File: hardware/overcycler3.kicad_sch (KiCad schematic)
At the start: 97 parts, among them J10 Control_Down, J2 AudioJack3_Switch, J3 DIN-5_180degree, J4 AudioJack3_Switch, J5 AudioJack3_Switch, J6 Control_Up, J7 Keyboard, J8 Display, J9 FT232, Q1 2SC945, SW1 RESET, U1 XT26G02CWSIGA, U2 TL064, U3 LPC1778FBD144, U4 TLV2556, U5 74HC138, U6 TL064, Y1 12MHz

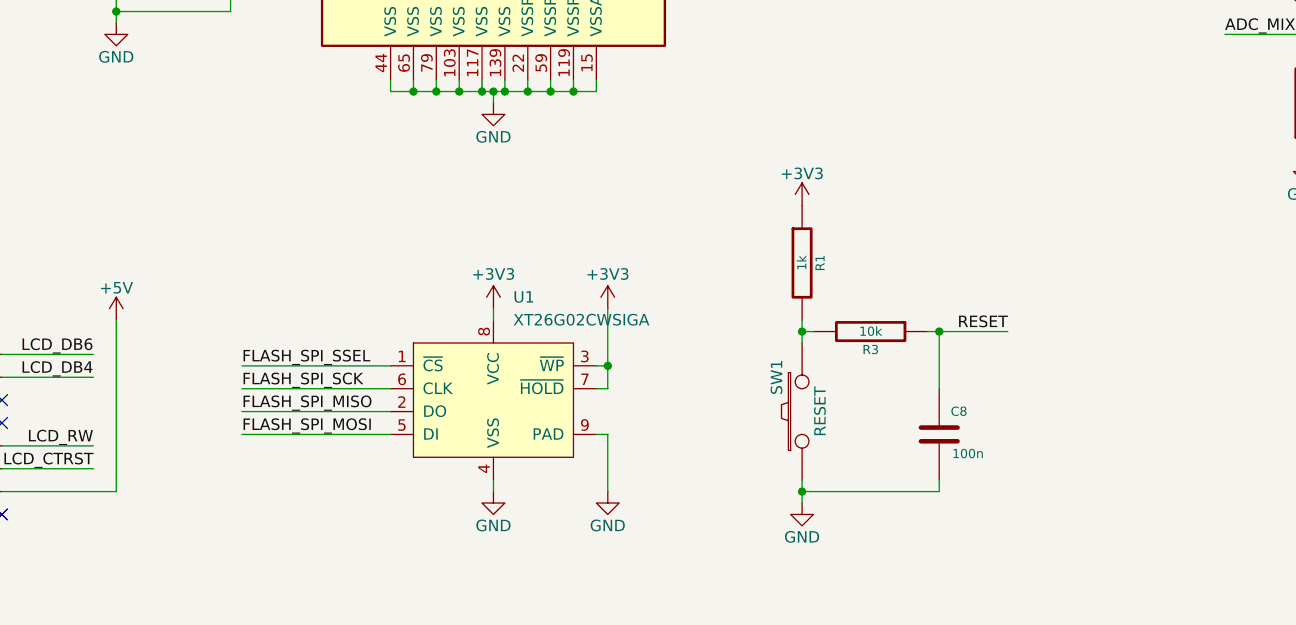
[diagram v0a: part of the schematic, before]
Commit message: sch: NAND -> 512Mb NOR FLASH
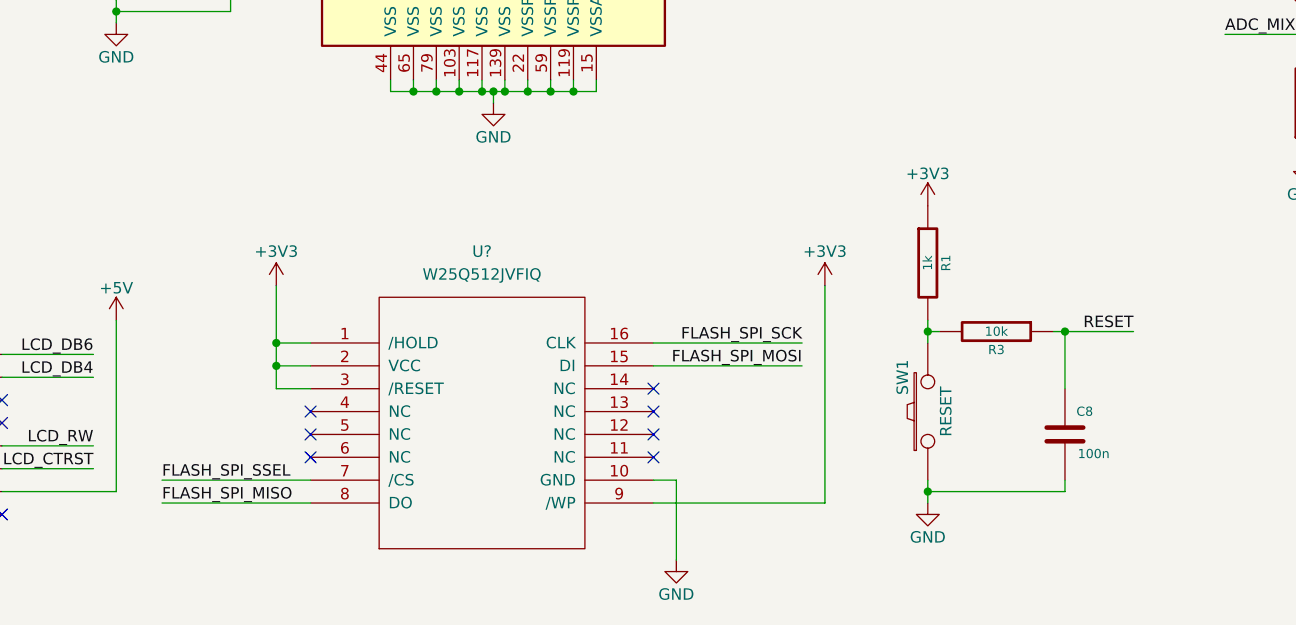
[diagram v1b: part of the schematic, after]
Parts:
- removed U1: XT26G02CWSIGA, Package_SON:WSON-8-1EP_8x6mm_P1.27mm_EP3.4x4.3mm, symbol Additional:XT26G02ELGIGA
- added U?: W25Q512JVFIQ, Package_SO:SOIC-16W_7.5x10.3mm_P1.27mm, symbol W25Q512JVFIQ:W25Q512JVFIQ
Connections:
- net +3V3: now also U?.1 (/HOLD), U?.2 (VCC), U?.3 (/RESET), U?.9 (/WP)
- net FLASH_SPI_MISO: now also U?.8 (DO)
- net FLASH_SPI_MOSI: now also U?.15 (DI)
- net FLASH_SPI_SCK: now also U?.16 (CLK)
- net FLASH_SPI_SSEL: now also U?.7 (/CS)
- net GND: now also U?.10 (GND)
- no-connect marks 99 -> 106
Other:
- moved on the sheet: C8, R1, R3, SW1
